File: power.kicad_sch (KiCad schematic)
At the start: 17 parts, among them Q1 XT60_YELLOW, U2 TPS56637RPAR

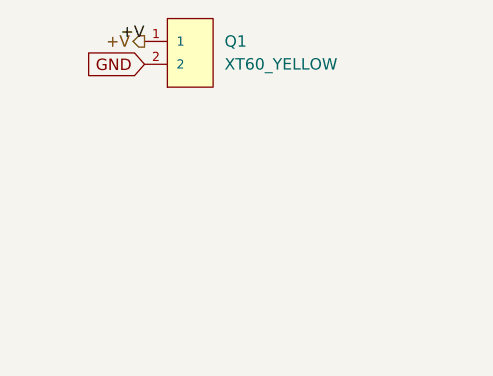
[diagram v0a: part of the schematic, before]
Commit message: idek
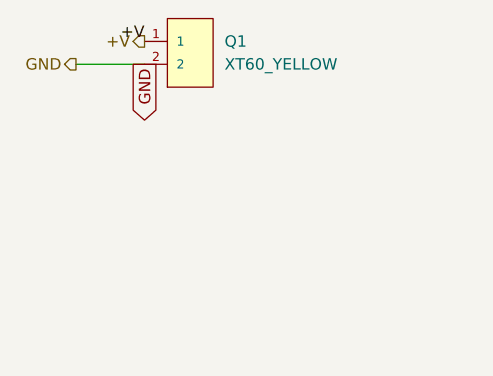
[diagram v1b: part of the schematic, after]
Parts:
- C1, C2, C3, C4, C5: footprint (none) -> Capacitor_SMD:C_1210_3225Metric
- L1: footprint (none) -> Inductor_SMD:L_1210_3225Metric
- R1, R2, R3, R4, R5, R6, R7, R8, R9: footprint (none) -> Resistor_SMD:R_0508_1220Metric
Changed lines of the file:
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@@
+	(wire
+		(pts
+			(xy 31.75 36.83) (xy 39.37 36.83)
+		)
+		(stroke
+			(width 0)
+			(type default)
+		)
+	)
 	(wire
 		(pts
@@
 	(global_label "GND"
 		(shape input)
-		(at 39.37 36.83 180)
+		(at 218.44 71.12 270)
 		(fields_autoplaced yes)
 		(effects
@@
 		)
 		(property "Intersheetrefs" "${INTERSHEET_REFS}"
-			(at 32.5143 36.83 0)
+			(at 218.44 77.9757 90)
 			(effects
 				(font
@@
 	(global_label "GND"
 		(shape input)
-		(at 218.44 71.12 270)
+		(at 113.03 74.93 270)
 		(fields_autoplaced yes)
 		(effects
@@
 		)
 		(property "Intersheetrefs" "${INTERSHEET_REFS}"
-			(at 218.44 77.9757 90)
+			(at 113.03 81.7857 90)
 			(effects
 				(font
@@
 	(global_label "GND"
 		(shape input)
-		(at 113.03 74.93 270)
+		(at 177.8 73.66 0)
 		(fields_autoplaced yes)
 		(effects
@@
 				(size 1.27 1.27)
 			)
-			(justify right)
+			(justify left)
 		)
 		(property "Intersheetrefs" "${INTERSHEET_REFS}"
-			(at 113.03 81.7857 90)
-			(effects
-				(font
-					(size 1.27 1.27)
-				)
-				(justify right)
+			(at 184.6557 73.66 0)
+			(effects
+				(font
+					(size 1.27 1.27)
+				)
+				(justify left)
 				(hide yes)
 			)
@@
 	(global_label "GND"
 		(shape input)
-		(at 177.8 73.66 0)
+		(at 123.19 74.93 270)
 		(fields_autoplaced yes)
 		(effects
@@
 				(size 1.27 1.27)
 			)
-			(justify left)
+			(justify right)
 		)
 		(property "Intersheetrefs" "${INTERSHEET_REFS}"
-			(at 184.6557 73.66 0)
-			(effects
-				(font
-					(size 1.27 1.27)
-				)
-				(justify left)
+			(at 123.19 81.7857 90)
+			(effects
+				(font
+					(size 1.27 1.27)
+				)
+				(justify right)
 				(hide yes)
 			)
@@
 	(global_label "GND"
 		(shape input)
-		(at 123.19 74.93 270)
+		(at 147.32 66.04 180)
 		(fields_autoplaced yes)
 		(effects
@@
 		)
 		(property "Intersheetrefs" "${INTERSHEET_REFS}"
-			(at 123.19 81.7857 90)
+			(at 140.4643 66.04 0)
 			(effects
 				(font
@@
 	)
 	(global_label "GND"
-		(shape input)
-		(at 147.32 66.04 180)
+		(shape output)
+		(at 39.37 36.83 270)
 		(fields_autoplaced yes)
 		(effects
@@
 		)
 		(property "Intersheetrefs" "${INTERSHEET_REFS}"
-			(at 140.4643 66.04 0)
+			(at 39.37 43.6857 90)
 			(effects
 				(font
@@
 			)
 			(justify left)
+		)
+	)
+	(hierarchical_label "GND"
+		(shape output)
+		(at 31.75 36.83 180)
+		(effects
+			(font
+				(size 1.27 1.27)
+			)
+			(justify right)
 		)
 	)
@@
 			)
 		)
-		(property "Footprint" ""
+		(property "Footprint" "Resistor_SMD:R_0508_1220Metric"
 			(at 121.412 71.12 90)
 			(effects
@@
 			)
 		)
-		(property "Footprint" ""
+		(property "Footprint" "Resistor_SMD:R_0508_1220Metric"
 			(at 225.552 69.85 90)
 			(effects
@@
 			)
 		)
-		(property "Footprint" ""
+		(property "Footprint" "Capacitor_SMD:C_1210_3225Metric"
 			(at 228.2952 66.04 0)
 			(effects
@@
 			)
 		)
-		(property "Footprint" ""
+		(property "Footprint" "Resistor_SMD:R_0508_1220Metric"
 			(at 209.55 57.658 90)
 			(effects
@@
 			)
 		)
-		(property "Footprint" ""
+		(property "Footprint" "Inductor_SMD:L_1210_3225Metric"
 			(at 189.23 53.34 0)
 			(effects
@@
 			)
 		)
-		(property "Footprint" ""
+		(property "Footprint" "Capacitor_SMD:C_1210_3225Metric"
 			(at 206.7052 63.5 0)
 			(effects
@@
 			)
 		)
-		(property "Footprint" ""
+		(property "Footprint" "Resistor_SMD:R_0508_1220Metric"
 			(at 181.61 67.818 90)
 			(effects
@@
 			)
 		)
-		(property "Footprint" ""
+		(property "Footprint" "Capacitor_SMD:C_1210_3225Metric"
 			(at 124.1552 67.31 0)
 			(effects
@@
 			)
 		)
-		(property "Footprint" ""
+		(property "Footprint" "Capacitor_SMD:C_1210_3225Metric"
 			(at 147.32 57.4548 0)
 			(effects
@@
 			)
 		)
-		(property "Footprint" ""
+		(property "Footprint" "Capacitor_SMD:C_1210_3225Metric"
 			(at 113.9952 67.31 0)
 			(effects
@@
 			)
 		)
-		(property "Footprint" ""
+		(property "Footprint" "Resistor_SMD:R_0508_1220Metric"
 			(at 220.218 57.15 90)
 			(effects
@@
 			)
 		)
-		(property "Footprint" ""
+		(property "Footprint" "Resistor_SMD:R_0508_1220Metric"
 			(at 111.252 71.12 90)
 			(effects
@@
 			)
 		)
-		(property "Footprint" ""
+		(property "Footprint" "Resistor_SMD:R_0508_1220Metric"
 			(at 135.89 60.198 90)
 			(effects
@@
 			)
 		)
-		(property "Footprint" ""
+		(property "Footprint" "Resistor_SMD:R_0508_1220Metric"
 			(at 220.218 67.31 90)
 			(effects
@@
 			)
 		)
-		(property "Footprint" ""
+		(property "Footprint" "Resistor_SMD:R_0508_1220Metric"
 			(at 196.85 55.118 90)
 			(effects
